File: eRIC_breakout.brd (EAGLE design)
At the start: 19.8 x 68.1 mm, 30 parts

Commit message: component values
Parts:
- C1: value (none) -> .1uF
- R1, R2: value (none) -> 10k
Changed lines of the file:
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@@
 <element name="SMA" library="SparkFun-Connectors" package="SMA-EDGE" value="" x="12.7" y="67.7"/>
 <element name="E$1" library="adafruit" package="1X12-CB" value="" x="26.7" y="19.85" rot="R90"/>
-<element name="C1" library="eagle-ltspice" package="C0603" value="" x="16.225" y="19.825" rot="MR90"/>
-<element name="R2" library="eagle-ltspice" package="R0402" value="" x="16.15" y="27" rot="MR90"/>
-<element name="R1" library="eagle-ltspice" package="R0402" value="" x="16.125" y="30.7" rot="MR270"/>
+<element name="C1" library="eagle-ltspice" package="C0603" value=".1uF" x="16.225" y="19.825" rot="MR90"/>
+<element name="R2" library="eagle-ltspice" package="R0402" value="10k" x="16.15" y="27" rot="MR90"/>
+<element name="R1" library="eagle-ltspice" package="R0402" value="10k" x="16.125" y="30.7" rot="MR270"/>
 </elements>
 <signals>

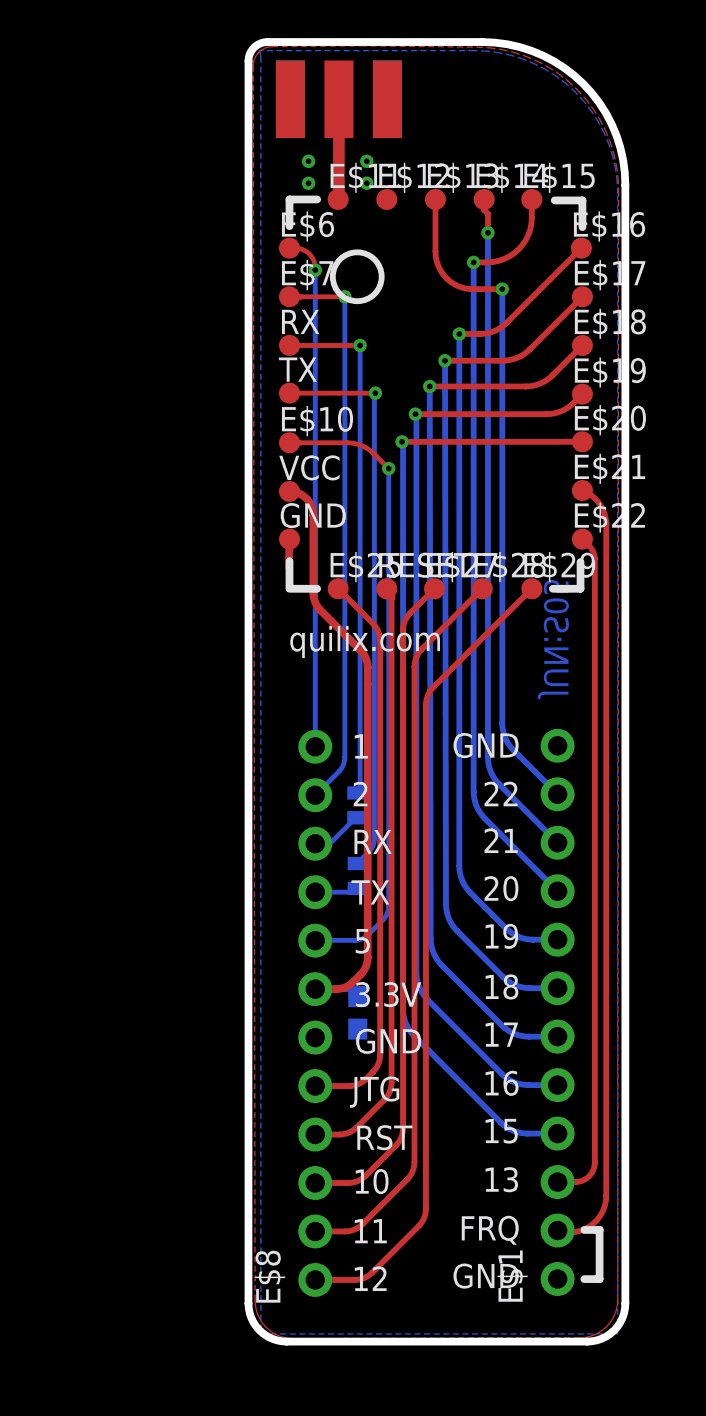
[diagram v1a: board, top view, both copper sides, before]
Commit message: overhaul of design, include schematic, un-tested
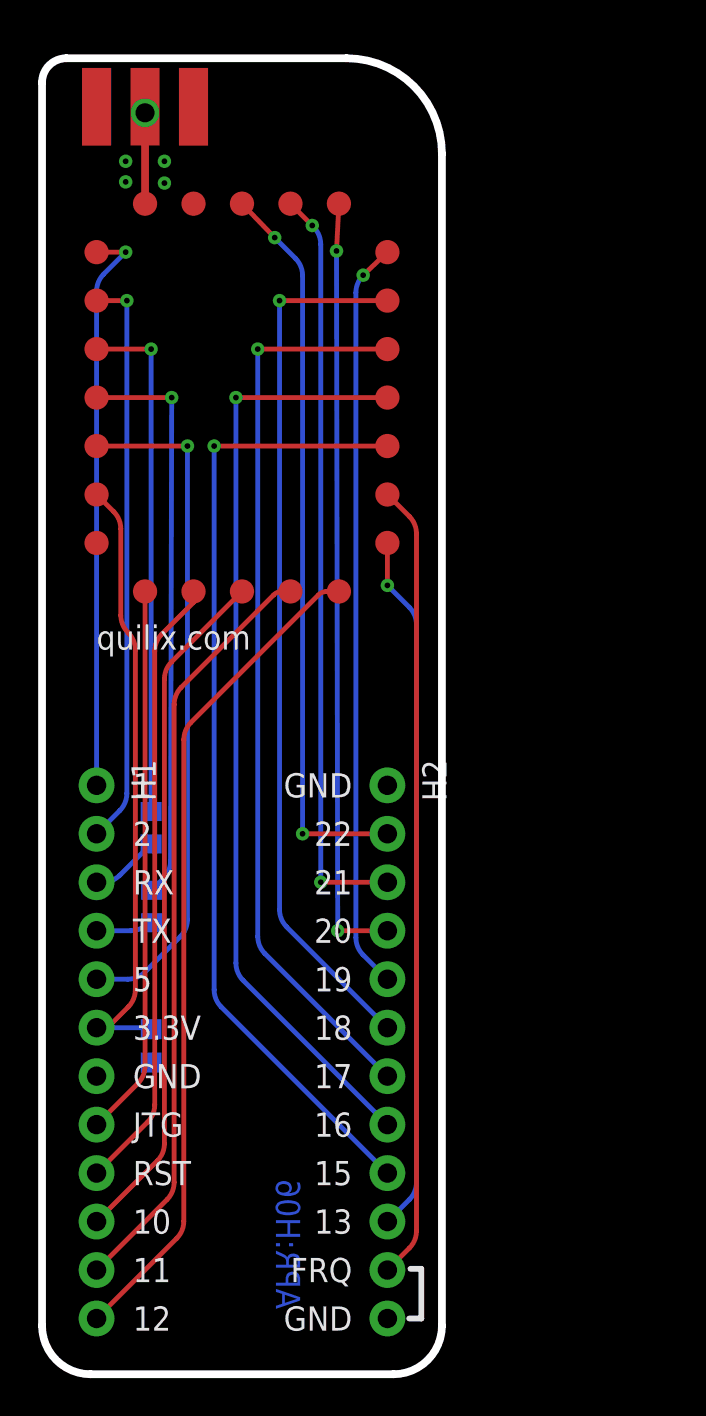
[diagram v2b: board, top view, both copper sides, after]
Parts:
- removed E$1, E$8: (no value), adafruit:1X12-CB
- removed E$10, E$11, E$12, E$13, E$14, E$15, E$16, E$17, E$18, E$19, E$20, E$21, E$22, E$25, E$27, E$28, E$29, E$6, E$7, GND, RESET, RX, TX, VCC: (no value), testpad:TP11R
- removed SMA: (no value), SparkFun-Connectors:SMA-EDGE
- added H1, H2: (no value), SparkFun-Connectors:1X12_NO_SILK_KIT
- added J$1: SMA_EDGE, SparkFun-Connectors:SMA-EDGE
- added U1: ERIC, lprs:ERIC
- C1: value .1uF -> (none); device eagle-ltspice:C0603 -> adafruit:C0603K
- R1, R2: value 10k -> (none); device eagle-ltspice:R0402 -> adafruit:R0603
- moved C1 11.0 mm to (5.40, 18.1)
- moved R2 10.8 mm to (5.42, 25.4), turned to 270 degrees
- moved R1 10.8 mm to (5.40, 29.5)
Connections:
- removed net S$1: C1.2, E$8.7, VCC.TP
- removed net S$10: E$6.TP, E$8.12
- removed net S$11: E$7.TP, E$8.11
- removed net S$12: E$10.TP, E$8.8
- removed net S$13: E$1.3, E$22.TP
- removed net S$14: E$1.2, E$21.TP
- removed net S$15: E$1.4, E$20.TP
- removed net S$16: E$1.5, E$19.TP
- removed net S$17: E$1.6, E$18.TP
- removed net S$18: E$1.7, E$17.TP
- removed net S$19: E$1.8, E$16.TP
- removed net S$2: R2.2, TX.TP
- removed net S$20: R1.1, RX.TP
- removed net S$21: E$28.TP, E$8.2
- removed net S$22: E$27.TP, E$8.3
- removed net S$23: E$25.TP, E$8.5
- removed net S$24: E$29.TP, E$8.1
- removed net S$25: E$11.TP, SMA.SIG
- removed net S$26: E$8.10, R1.2
- removed net S$3: E$8.4, RESET.TP
- removed net S$4: E$8.9, R2.1
- removed net S$6: E$1.11, E$13.TP
- removed net S$7: E$1.10, E$14.TP
- removed net S$9: E$1.9, E$15.TP
- new net N$1: H1.1, U1.CD
- new net N$11: H1.8, U1.E8
- new net N$12: H1.9, U1.E9
- new net N$13: H1.10, U1.E10
- new net N$14: H1.11, U1.E11
- new net N$15: H1.12, U1.E12
- new net N$16: H2.9, U1.E15
- new net N$17: H2.8, U1.E16
- new net N$18: H2.7, U1.E17
- new net N$19: H2.6, U1.E18
- new net N$2: H1.2, U1.BUSY
- new net N$20: H2.5, U1.E19
- new net N$21: H2.4, U1.E20
- new net N$22: H2.3, U1.E21
- new net N$23: H2.2, U1.E22
- new net N$24: H2.11, U1.FS
- new net N$25: H2.10, U1.E13
- new net N$3: J$1.SIG, U1.ANT
- new net N$8: H1.5, U1.HR
- new net SDI: H1.4, R2.1, R2.2, U1.SDI
- new net SDO: H1.3, R1.1, R1.2, U1.SDO
- new net VCC: C1.2, H1.6, U1.VCC
- net GND: now also H1.7, H2.1, H2.12, J$1.GND@0, J$1.GND@1, J$1.GND@2, J$1.GND@3, U1.AGND, U1.GND; no longer E$1.1, E$1.12, E$12.TP, E$8.6, GND.TP, SMA.GND@0, SMA.GND@1, SMA.GND@2, SMA.GND@3
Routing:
- net N$16: track 0.00 -> 50.9 mm, vias 0 -> 1
- net S$15: track 50.2 -> 0.00 mm, vias 1 -> 0
- net N$17: track 0.00 -> 49.2 mm, vias 0 -> 1
- net S$16: track 48.4 -> 0.00 mm, vias 1 -> 0
- net N$18: track 0.00 -> 47.6 mm, vias 0 -> 1
- net S$17: track 46.7 -> 0.00 mm, vias 1 -> 0
- net N$19: track 0.00 -> 46.0 mm, vias 0 -> 1
- net S$18: track 44.9 -> 0.00 mm, vias 1 -> 0
- net N$15: track 0.00 -> 43.7 mm
- net S$19: track 43.0 -> 0.00 mm, vias 1 -> 0
- net S$24: track 42.2 -> 0.00 mm
- net N$24: track 0.00 -> 41.7 mm
- net N$21: track 0.00 -> 40.7 mm, vias 0 -> 2
- net S$14: track 40.5 -> 0.00 mm
- net N$14: track 0.00 -> 40.0 mm
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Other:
- board size 19.8 x 68.1 mm -> 21 x 69 mm
- board text added: "APR:H06"
- board text removed: "JUN:S05"
